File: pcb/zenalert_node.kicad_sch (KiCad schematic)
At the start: 14 parts, among them J1 MQ135 (Air Quality), J2 MQ2 (Gas / Smoke), J3 DHT22 (Temp & Hum), J4 SSD1306 OLED (I2C), J5 I2C Expansion, U1 ESP32-S2-Mini

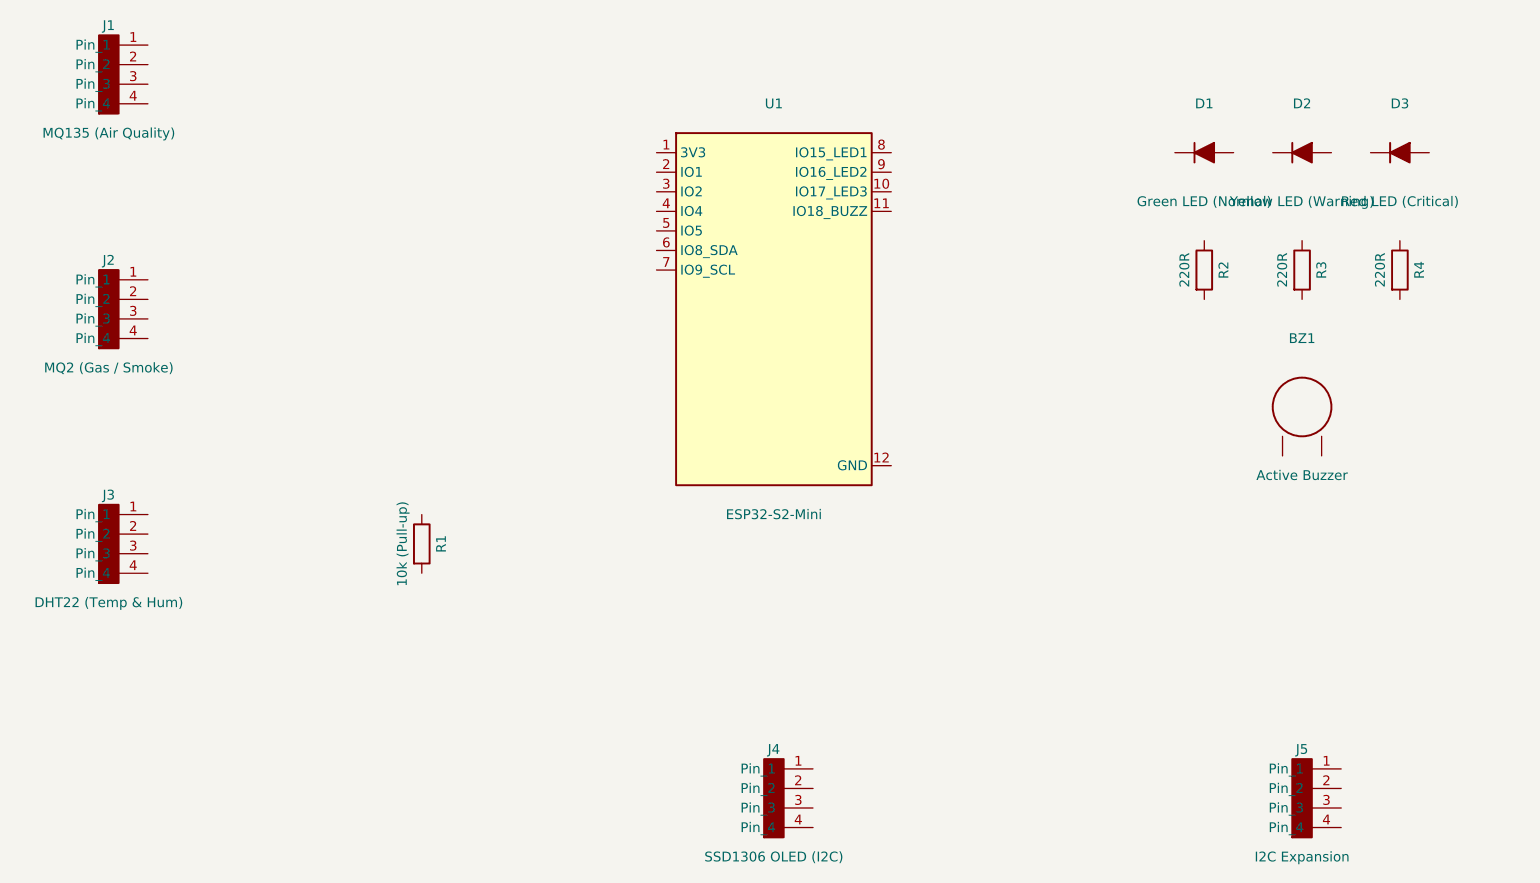
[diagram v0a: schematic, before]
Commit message: feat (pcb) : add kicad design files production gerber and hardware documentation
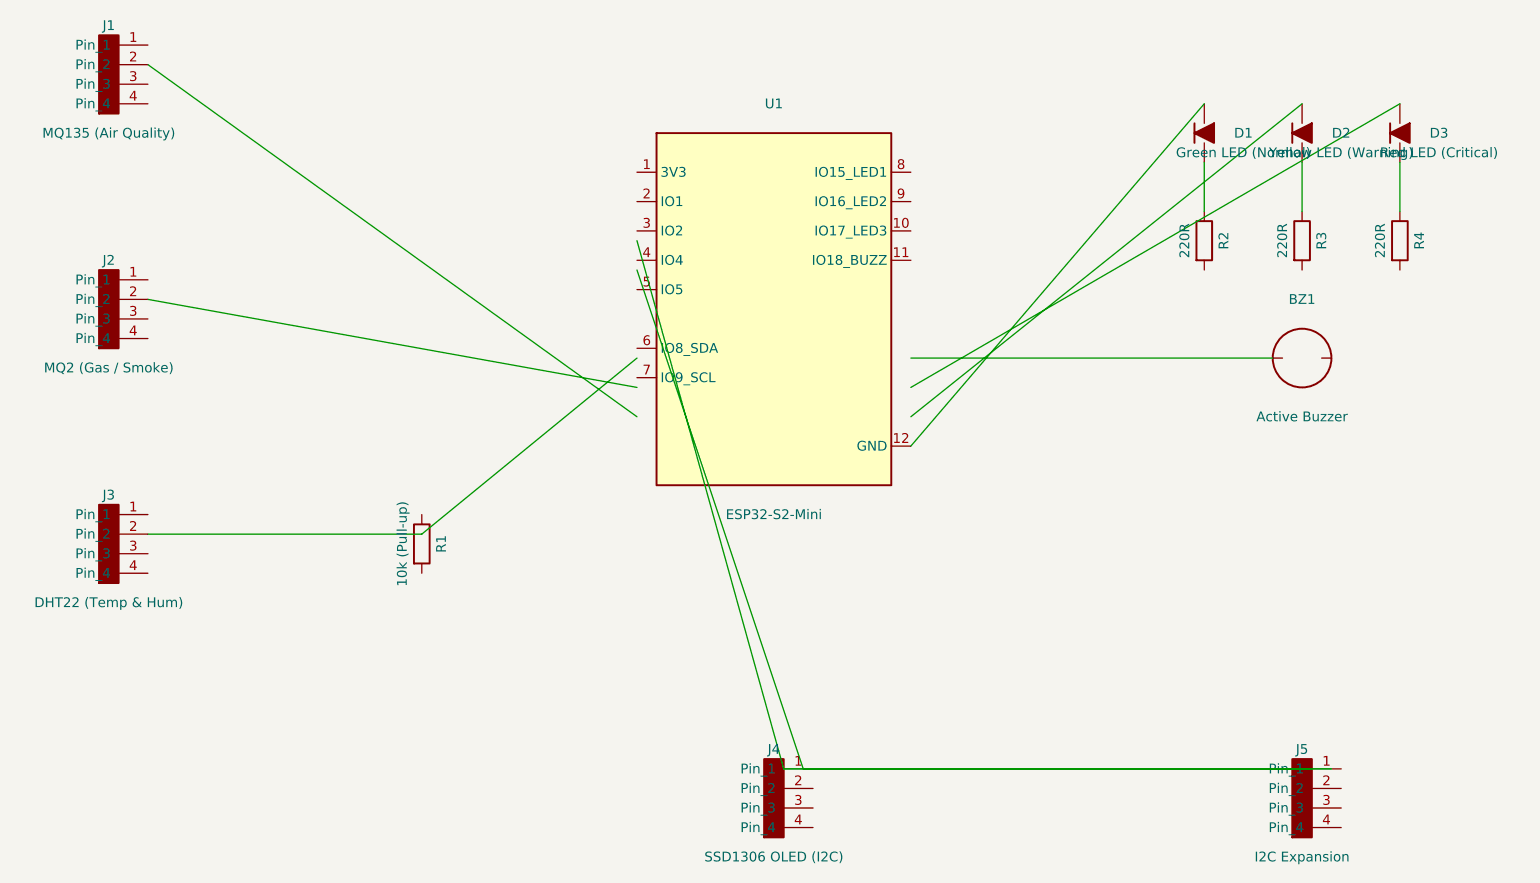
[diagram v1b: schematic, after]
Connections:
- net at U1.12 (GND): now also D1.1 (A)
- net at D1.2 (K): now also R2.1
- net at D2.2 (K): now also R3.1
- net at D3.2 (K): now also R4.1
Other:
- moved on the sheet: BZ1, D1, D2, D3, R2, R3, R4
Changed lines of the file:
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@@
     (property "Value" "I2C Expansion" (at 215.9 172.72 0))
   )
-  (symbol (lib_id "Device:LED") (at 203.2 81.28 0) (unit 1)
+  (symbol (lib_id "Device:LED") (at 203.2 78.74 0) (unit 1)
     (in_bom yes) (on_board yes) (dnp no)
-    (property "Reference" "D1" (at 203.2 74.93 0))
-    (property "Value" "Green LED (Normal)" (at 203.2 87.63 0))
+    (property "Reference" "D1" (at 208.28 78.74 0))
+    (property "Value" "Green LED (Normal)" (at 208.28 81.28 0))
   )
-  (symbol (lib_id "Device:LED") (at 215.9 81.28 0) (unit 1)
+  (symbol (lib_id "Device:LED") (at 215.9 78.74 0) (unit 1)
     (in_bom yes) (on_board yes) (dnp no)
-    (property "Reference" "D2" (at 215.9 74.93 0))
-    (property "Value" "Yellow LED (Warning)" (at 215.9 87.63 0))
+    (property "Reference" "D2" (at 220.98 78.74 0))
+    (property "Value" "Yellow LED (Warning)" (at 220.98 81.28 0))
   )
-  (symbol (lib_id "Device:LED") (at 228.6 81.28 0) (unit 1)
+  (symbol (lib_id "Device:LED") (at 228.6 78.74 0) (unit 1)
     (in_bom yes) (on_board yes) (dnp no)
-    (property "Reference" "D3" (at 228.6 74.93 0))
-    (property "Value" "Red LED (Critical)" (at 228.6 87.63 0))
+    (property "Reference" "D3" (at 233.68 78.74 0))
+    (property "Value" "Red LED (Critical)" (at 233.68 81.28 0))
   )
-  (symbol (lib_id "Device:Buzzer") (at 215.9 114.3 0) (unit 1)
+  (symbol (lib_id "Device:Buzzer") (at 215.9 107.95 0) (unit 1)
     (in_bom yes) (on_board yes) (dnp no)
-    (property "Reference" "BZ1" (at 215.9 105.41 0))
-    (property "Value" "Active Buzzer" (at 215.9 123.19 0))
+    (property "Reference" "BZ1" (at 215.9 100.33 0))
+    (property "Value" "Active Buzzer" (at 215.9 115.57 0))
   )
   (symbol (lib_id "Device:R") (at 101.6 132.08 0) (unit 1)
@@
     (property "Value" "10k (Pull-up)" (at 99.06 132.08 90))
   )
-  (symbol (lib_id "Device:R") (at 203.2 96.52 0) (unit 1)
+  (symbol (lib_id "Device:R") (at 203.2 92.71 0) (unit 1)
     (in_bom yes) (on_board yes) (dnp no)
-    (property "Reference" "R2" (at 205.74 96.52 90))
-    (property "Value" "220R" (at 200.66 96.52 90))
+    (property "Reference" "R2" (at 205.74 92.71 90))
+    (property "Value" "220R" (at 200.66 92.71 90))
   )
-  (symbol (lib_id "Device:R") (at 215.9 96.52 0) (unit 1)
+  (symbol (lib_id "Device:R") (at 215.9 92.71 0) (unit 1)
     (in_bom yes) (on_board yes) (dnp no)
-    (property "Reference" "R3" (at 218.44 96.52 90))
-    (property "Value" "220R" (at 213.36 96.52 90))
+    (property "Reference" "R3" (at 218.44 92.71 90))
+    (property "Value" "220R" (at 213.36 92.71 90))
   )
-  (symbol (lib_id "Device:R") (at 228.6 96.52 0) (unit 1)
+  (symbol (lib_id "Device:R") (at 228.6 92.71 0) (unit 1)
     (in_bom yes) (on_board yes) (dnp no)
-    (property "Reference" "R4" (at 231.14 96.52 90))
-    (property "Value" "220R" (at 226.06 96.52 90))
+    (property "Reference" "R4" (at 231.14 92.71 90))
+    (property "Value" "220R" (at 226.06 92.71 90))
   )
+  (wire (pts (xy 66.04 69.85) (xy 129.54 115.57)))
+  (wire (pts (xy 66.04 100.33) (xy 129.54 111.76)))
+  (wire (pts (xy 66.04 130.81) (xy 101.6 130.81)))
+  (wire (pts (xy 101.6 130.81) (xy 129.54 107.95)))
+  (wire (pts (xy 165.1 119.38) (xy 203.2 74.93)))
+  (wire (pts (xy 165.1 115.57) (xy 215.9 74.93)))
+  (wire (pts (xy 165.1 111.76) (xy 228.6 74.93)))
+  (wire (pts (xy 165.1 107.95) (xy 212.09 107.95)))
+  (wire (pts (xy 203.2 82.55) (xy 203.2 88.9)))
+  (wire (pts (xy 215.9 82.55) (xy 215.9 88.9)))
+  (wire (pts (xy 228.6 82.55) (xy 228.6 88.9)))
+  (wire (pts (xy 129.54 96.52) (xy 151.13 161.29)))
+  (wire (pts (xy 129.54 92.71) (xy 148.59 161.29)))
+  (wire (pts (xy 151.13 161.29) (xy 219.71 161.29)))
+  (wire (pts (xy 148.59 161.29) (xy 217.17 161.29)))
   (sheet_instances
     (path "/" (page "1"))
